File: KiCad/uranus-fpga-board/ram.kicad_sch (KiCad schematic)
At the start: 62 parts, among them U2 NT5CB64M16GP-FL, U3 NT5CB64M16GP-FL, U4 NT5CB64M16GP-FL, U5 NT5CB64M16GP-FL, Y1 SX7DF200.000B20F30DNN

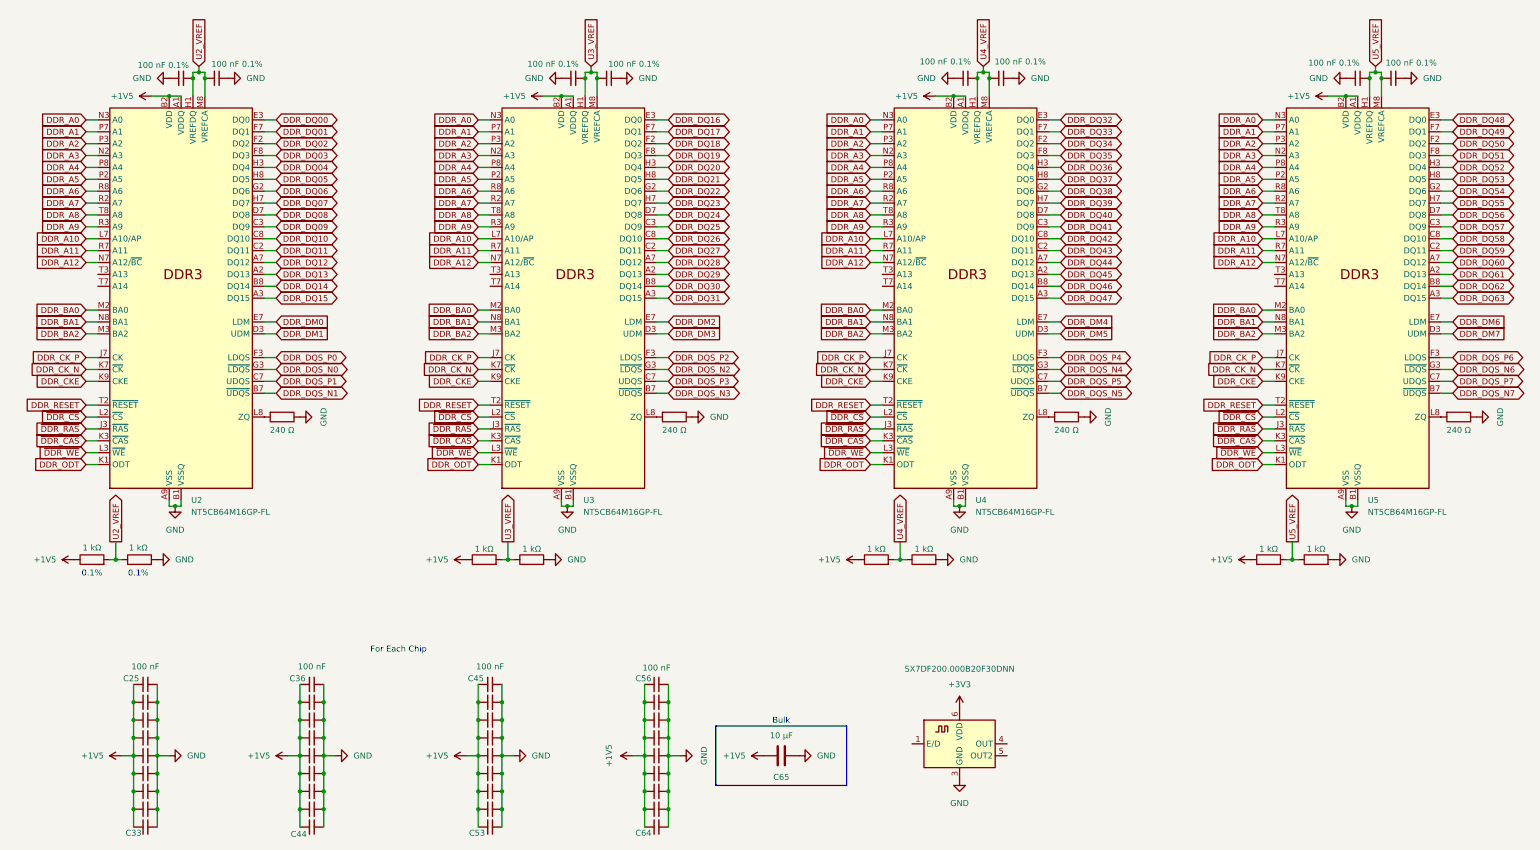
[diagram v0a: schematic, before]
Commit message: big things happening in schematic quality
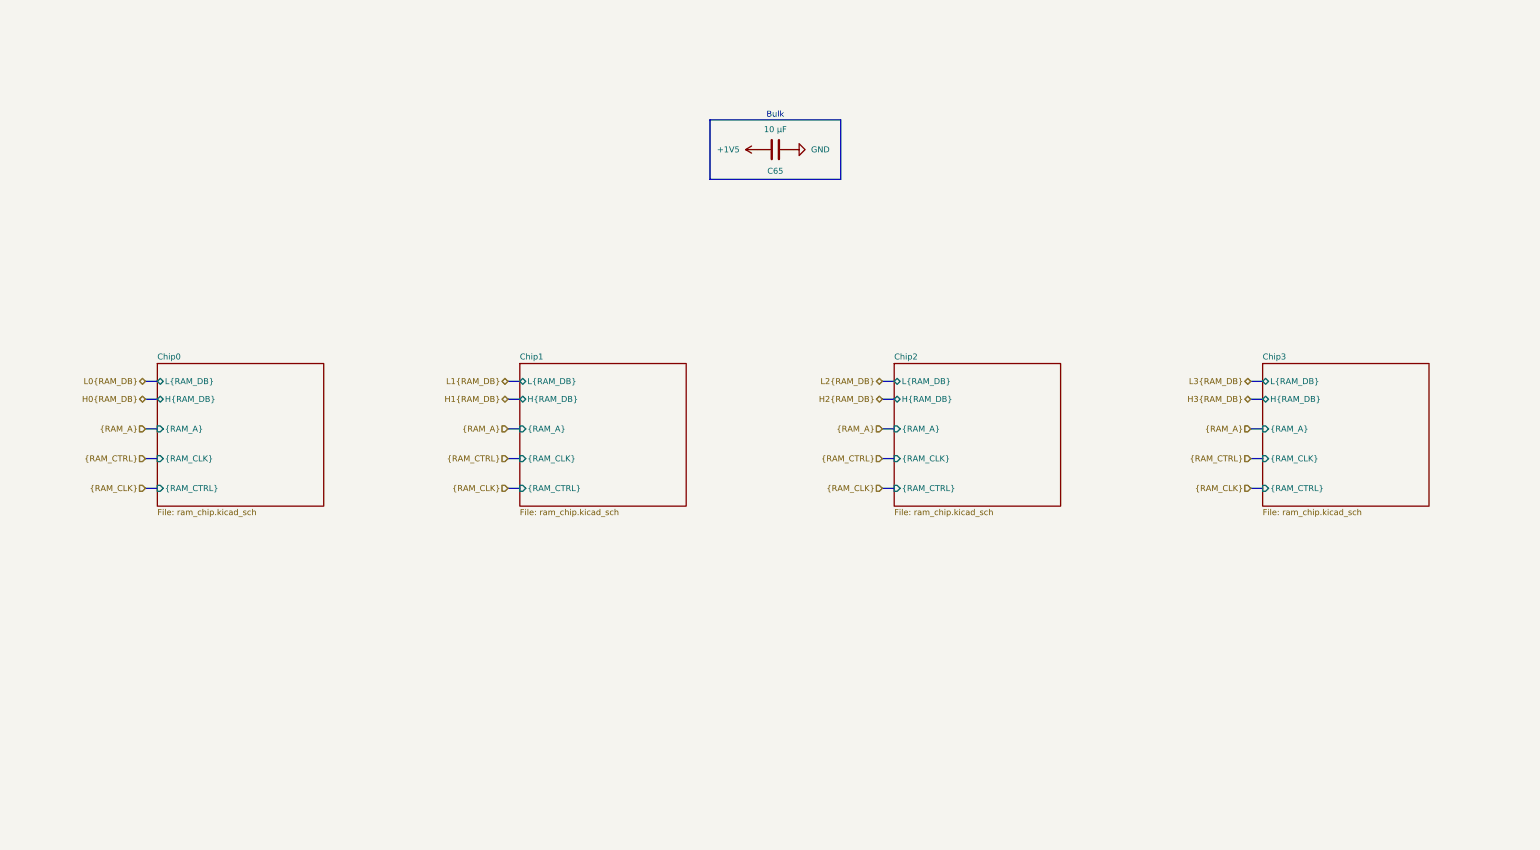
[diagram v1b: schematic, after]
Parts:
- removed C25, C26, C27, C28, C29, C30, C31, C32, C33, C36, C37, C38, C39, C40, C41, C42, C43, C44, C45, C46, C47, C48, C49, C50, C51, C52, C53, C56, C57, C58, C59, C60, C61, C62, C63, C64: 100 nF, symbol Device:C_Small
- removed C34, C35, C54, C55, C66, C67, C68, C69: 100 nF 0.1%, symbol Device:C_Small
- removed R1, R10, R11, R2, R4, R5, R7, R8: 1 kΩ, Resistor_SMD:R_0402_1005Metric, symbol Device:R
- removed R12, R3, R6, R9: 240 Ω, Resistor_SMD:R_0402_1005Metric, symbol Device:R
- removed U2, U3, U4, U5: NT5CB64M16GP-FL, Package_BGA:FBGA-96_8x13mm_Layout9x16_P0.8mm, symbol Memory_RAM:AS4C256M16D3
- removed Y1: SX7DF200.000B20F30DNN, Oscillator:Oscillator_SMD_IDT_JU6-6_7.0x5.0mm_P2.54mm, symbol Oscillator:XUX71
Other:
- added sheet Chip0 (ram_chip.kicad_sch)
- added sheet Chip1 (ram_chip.kicad_sch)
- added sheet Chip2 (ram_chip.kicad_sch)
- added sheet Chip3 (ram_chip.kicad_sch)
- note removed: "0.1%"
- note removed: "For Each Chip"
- moved on the sheet: C65

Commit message: Big things have mostly happened in schematic quality
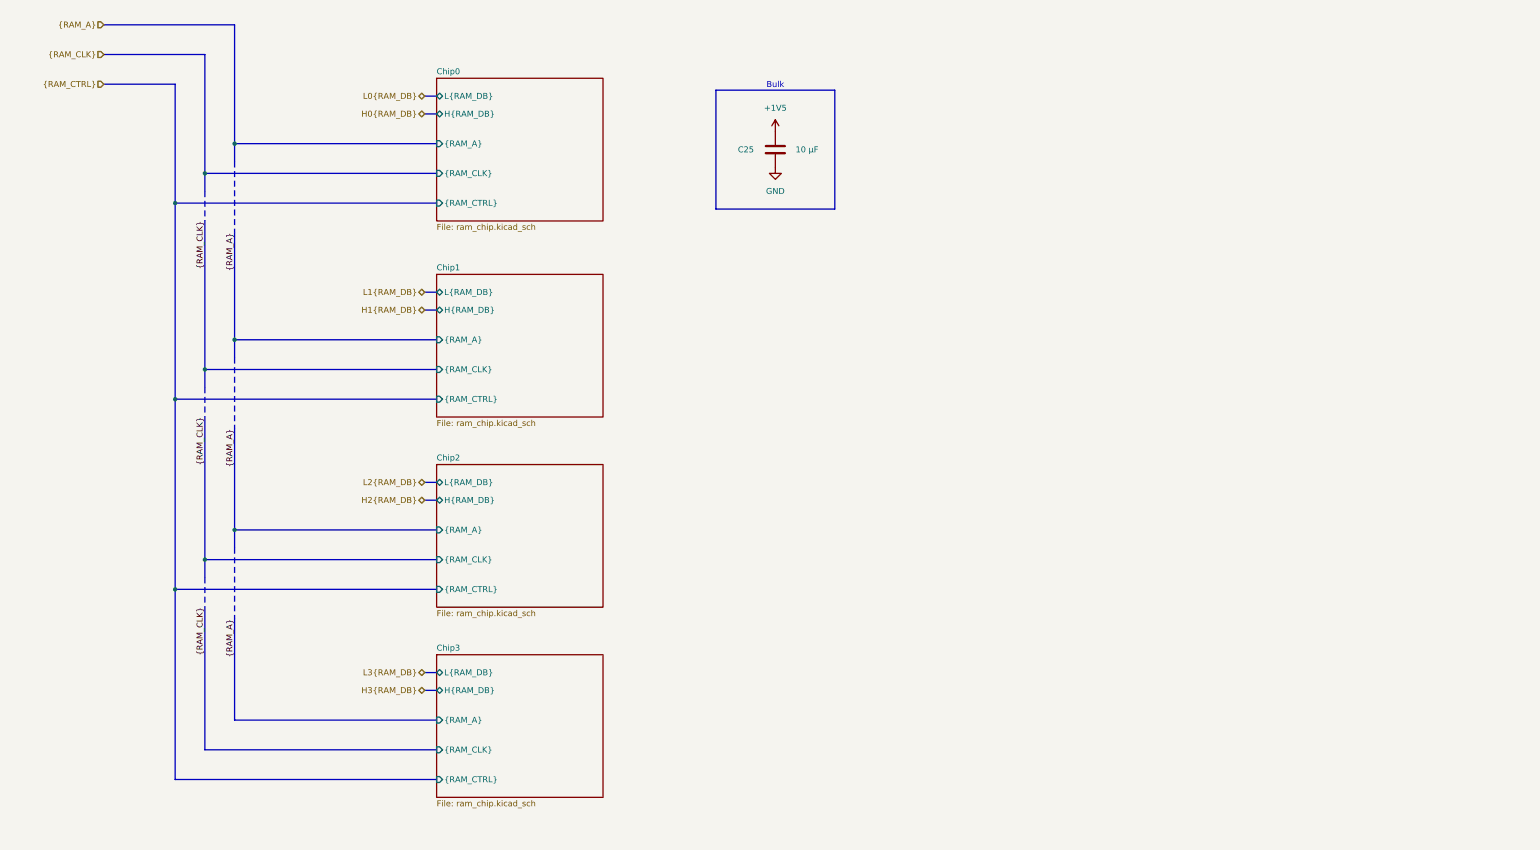
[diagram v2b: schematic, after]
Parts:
- renumbered C65 to C25
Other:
- moved on the sheet: C25
